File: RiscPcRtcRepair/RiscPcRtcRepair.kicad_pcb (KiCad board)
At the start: 2 copper layers, 22.5 x 32 mm, 16 parts, among them U1 PCF8583T, Y1 Crystal_GND3

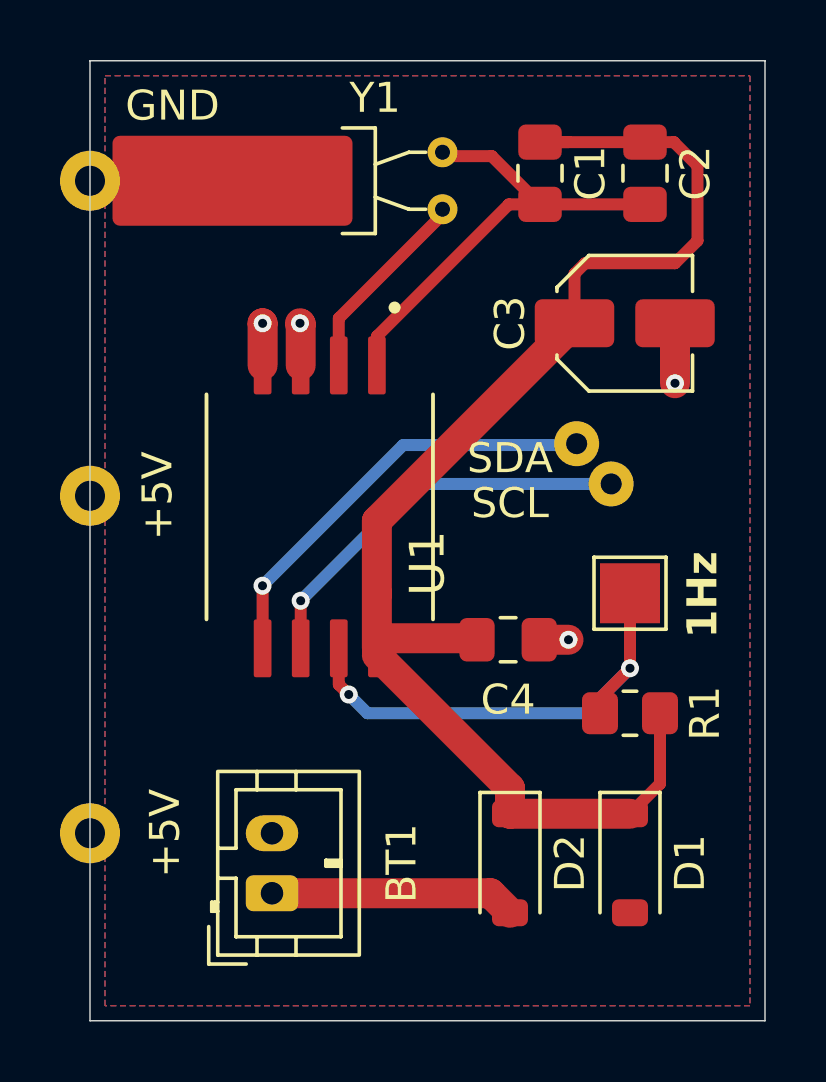
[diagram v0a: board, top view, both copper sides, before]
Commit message: Fix warnings and add gerbers
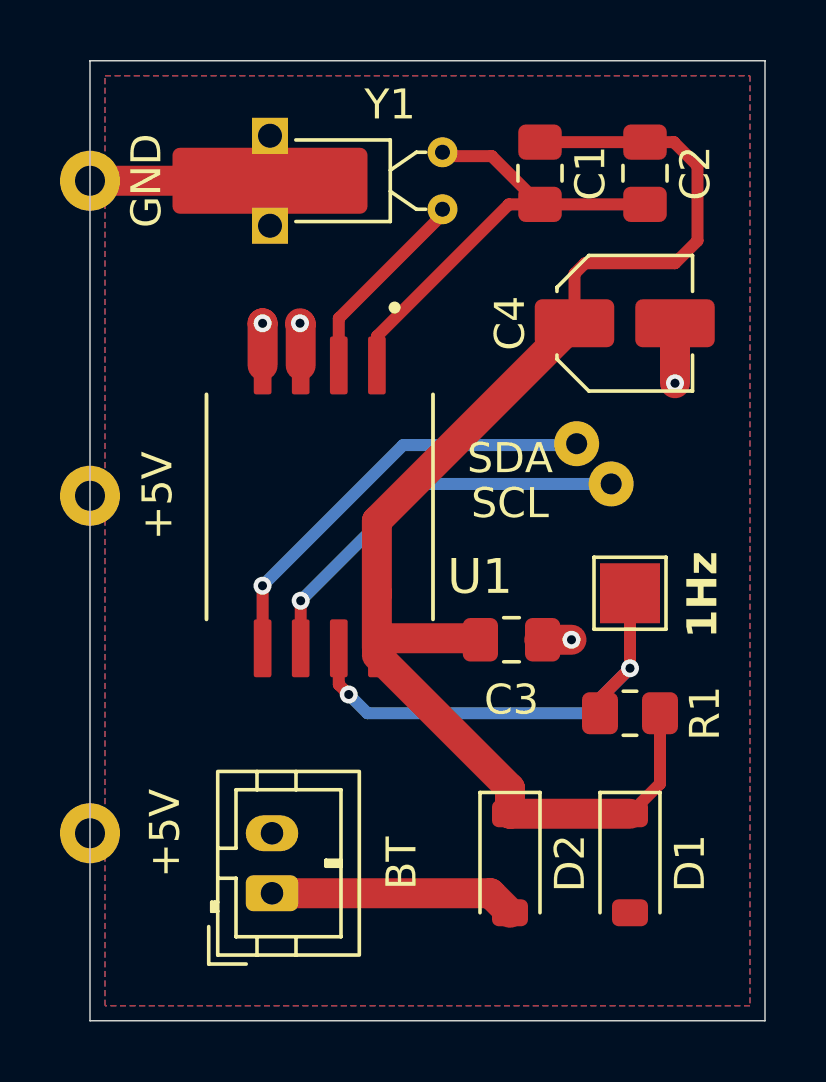
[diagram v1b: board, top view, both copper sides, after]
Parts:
- Y1: footprint Crystal:Crystal_C38-LF_D3.0mm_L8.0mm_Horizontal_1EP_style1 -> Crystal:Crystal_C26-LF_D2.1mm_L6.5mm_Horizontal_1EP_style2
- moved C3 0.11 mm to (107.0, 86.0)
- renumbered +5V2 to +5V1, BT1 to BT, C4 to C3, C3 to C4
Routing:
- net GND: track 5.80 -> 11.1 mm
- net Net-(D1-K): track 48.2 -> 47.2 mm
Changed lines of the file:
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@@
 		(tags "test point THT pad")
 		(property "Reference" "GND"
-			(at 2.75 -2.5 0)
+			(at 1.881715 0 90)
 			(layer "F.SilkS")
 			(effects
@@
 			(pinfunction "1")
 			(pintype "passive")
+			(zone_connect 2)
 		)
 		(embedded_fonts no)
@@
 		(descr "SMD capacitor, aluminum electrolytic nonpolar, 4.0x5.4mm")
 		(tags "capacitor electrolytic nonpolar")
-		(property "Reference" "C3"
+		(property "Reference" "C4"
 			(at -3.825 0 90)
 			(layer "F.SilkS")
@@
 		)
 	)
-	(footprint "Crystal:Crystal_C38-LF_D3.0mm_L8.0mm_Horizontal_1EP_style1"
+	(footprint "Crystal:Crystal_C26-LF_D2.1mm_L6.5mm_Horizontal_1EP_style2"
 		(layer "F.Cu")
 		(at 104.75 69.8 -90)
-		(descr "C38-LF, Crystal, length 8.0mm, width 3.0mm, THT")
+		(descr "C26-LF, Crystal, length 6.5mm, width 2.1mm, THT")
 		(property "Reference" "Y1"
-			(at -1.81 2.25 0)
+			(at -1.59 1.75 0)
 			(layer "F.SilkS")
 			(effects
@@
 		)
 		(property "Value" "Crystal_GND3"
-			(at 3.71 2.25 0)
+			(at 3.49 1.75 0)
 			(layer "F.Fab")
 			(effects
@@
 			)
 		)
-		(property "Datasheet" "~"
-			(at 0 0 90)
+		(property "Datasheet" ""
+			(at 0 0 270)
 			(layer "F.Fab")
 			(hide yes)
@@
 			)
 		)
-		(property "Description" "Three pin crystal, GND on pin 3"
-			(at 0 0 90)
+		(property "Description" ""
+			(at 0 0 270)
 			(layer "F.Fab")
 			(hide yes)
@@
 		(attr through_hole)
 		(fp_line
-			(start -0.81 3.34)
-			(end -0.81 2.24)
+			(start -0.41 4.89)
+			(end -0.41 1.74)
 			(stroke
 				(width 0.12)
@@
 		)
 		(fp_line
-			(start -0.81 2.24)
-			(end 2.71 2.24)
+			(start -0.41 1.74)
+			(end 2.31 1.74)
 			(stroke
 				(width 0.12)
@@
 		)
 		(fp_line
-			(start 0.405 2.24)
-			(end 0 1.12)
+			(start 0.6 1.74)
+			(end 0 0.87)
 			(stroke
 				(width 0.12)
@@
 		)
 		(fp_line
-			(start 1.495 2.24)
-			(end 1.9 1.12)
+			(start 1.3 1.74)
+			(end 1.9 0.87)
 			(stroke
 				(width 0.12)
@@
 		)
 		(fp_line
-			(start 2.71 2.24)
-			(end 2.71 3.34)
+			(start 2.31 1.74)
+			(end 2.31 4.89)
 			(stroke
 				(width 0.12)
@@
 		)
 		(fp_line
-			(start 0 1.12)
+			(start 0 0.87)
 			(end 0 0.56)
 			(stroke
@@
 		)
 		(fp_line
-			(start 1.9 1.12)
+			(start 1.9 0.87)
 			(end 1.9 0.56)
 			(stroke
@@
 		)
 		(fp_rect
-			(start -1.3 -0.75)
-			(end 3.2 11.25)
+			(start -1.4 -0.75)
+			(end 3.3 9.25)
 			(stroke
 				(width 0.05)
@@
 		)
 		(fp_line
-			(start 0.405 2.5)
-			(end 0 1.25)
+			(start -0.55 5.75)
+			(end 2.45 5.75)
 			(stroke
 				(width 0.1)
@@
 		)
 		(fp_line
-			(start 1.495 2.5)
-			(end 1.9 1.25)
+			(start 0.6 2)
+			(end 0 1)
 			(stroke
 				(width 0.1)
@@
 		)
 		(fp_line
-			(start 0 1.25)
+			(start 1.3 2)
+			(end 1.9 1)
+			(stroke
+				(width 0.1)
+				(type solid)
+			)
+			(layer "F.Fab")
+		)
+		(fp_line
+			(start 0 1)
 			(end 0 0)
 			(stroke
@@
 		)
 		(fp_line
-			(start 1.9 1.25)
+			(start 1.9 1)
 			(end 1.9 0)
 			(stroke
@@
 		)
 		(fp_rect
-			(start -0.55 2.5)
-			(end 2.45 10.5)
+			(start -0.08 2)
+			(end 1.98 8.5)
 			(stroke
 				(width 0.1)
@@
 		)
 		(fp_text user "${REFERENCE}"
-			(at 0.95 6.45 0)
+			(at 0.95 5.25 0)
 			(layer "F.Fab")
 			(effects
@@
 			(pintype "passive")
 		)
+		(pad "3" thru_hole rect
+			(at -0.55 5.75 270)
+			(size 1.2 1.2)
+			(drill 0.8)
+			(layers "*.Cu" "*.Mask")
+			(remove_unused_layers no)
+			(net 2 "GND")
+			(pinfunction "3")
+			(pintype "passive")
+		)
 		(pad "3" smd roundrect
-			(at 0.95 7 270)
-			(size 3 8)
+			(at 0.95 5.75 270)
+			(size 2.2 6.5)
 			(layers "F.Cu" "F.Mask" "F.Paste")
-			(roundrect_rratio 0.083333)
+			(roundrect_rratio 0.113636)
+			(net 2 "GND")
+			(pinfunction "3")
+			(pintype "passive")
+		)
+		(pad "3" thru_hole rect
+			(at 2.45 5.75 270)
+			(size 1.2 1.2)
+			(drill 0.8)
+			(layers "*.Cu" "*.Mask")
+			(remove_unused_layers no)
 			(net 2 "GND")
 			(pinfunction "3")
@@
 		)
 		(embedded_fonts no)
-		(model "${KICAD9_3DMODEL_DIR}/Crystal.3dshapes/Crystal_C38-LF_D3.0mm_L8.0mm_Horizontal_1EP_style1.step"
+		(model "${KICAD9_3DMODEL_DIR}/Crystal.3dshapes/Crystal_C26-LF_D2.1mm_L6.5mm_Horizontal_1EP_style2.step"
 			(offset
 				(xyz 0 0 0)
@@
 		(descr "JST PH series connector, B2B-PH-K (http://www.jst-mfg.com/product/pdf/eng/ePH.pdf), generated with kicad-footprint-generator")
 		(tags "connector JST PH vertical")
-		(property "Reference" "BT1"
+		(property "Reference" "BT"
 			(at 1 4.318777 90)
 			(layer "F.SilkS")
@@
 			(pinfunction "-")
 			(pintype "passive")
+			(zone_connect 2)
 		)
 		(embedded_fonts no)
@@
 		(descr "THT pad as test Point, diameter 2.0mm, hole diameter 1.0mm")
 		(tags "test point THT pad")
-		(property "Reference" "+5V2"
+		(property "Reference" "+5V1"
 			(at 1.5 -3 90)
 			(layer "F.SilkS")
@@
 		(at 100.658166 81.620968 -90)
 		(property "Reference" "U1"
-			(at 1.879032 -3.591834 270)
+			(at 2.329032 -5.341834 0)
 			(layer "F.SilkS")
 			(effects
@@
 	(footprint "Capacitor_SMD:C_0805_2012Metric_Pad1.18x1.45mm_HandSolder"
 		(layer "F.Cu")
-		(at 106.9375 86.05 180)
+		(at 107.05 86.05 180)
 		(descr "Capacitor SMD 0805 (2012 Metric), square (rectangular) end terminal, IPC-7351 nominal with elongated pad for handsoldering. (Body size source: IPC-SM-782 page 76, https://www.pcb-3d.com/wordpress/wp-content/uploads/ipc-sm-782a_amendment_1_and_2.pdf, https://docs.google.com/spreadsheets/d/1BsfQQcO9C6DZCsRaXUlFlo91Tg2WpOkGARC1WS5S8t0/edit?usp=sharing), generated with kicad-footprint-generator")
 		(tags "capacitor handsolder")
-		(property "Reference" "C4"
+		(property "Reference" "C3"
 			(at 0 -2 0)
 			(layer "F.SilkS")
@@
 	)
 	(segment
-		(start 100.023166 76.905968)
-		(end 100.023166 75.523166)
+		(start 107.975 86.05)
+		(end 109.05 86.05)
 		(width 1)
 		(layer "F.Cu")
@@
 	)
 	(segment
-		(start 107.975 86.05)
-		(end 108.95 86.05)
+		(start 99 70.75)
+		(end 93.8 70.75)
+		(width 1)
+		(layer "F.Cu")
+		(net 2)
+	)
+	(segment
+		(start 100.023166 76.905968)
+		(end 100.023166 75.523166)
 		(width 1)
 		(layer "F.Cu")
@@
 	)
 	(via
-		(at 108.95 86.05)
+		(at 100 75.5)
 		(size 0.6)
 		(drill 0.3)
@@
 	)
 	(via
-		(at 100 75.5)
+		(at 109.05 86.05)
 		(size 0.6)
 		(drill 0.3)
@@
 	(segment
 		(start 102.563166 82.086834)
-		(end 109.15 75.5)
+		(end 102.563166 84.5)
 		(width 1)
 		(layer "F.Cu")
@@
 	)
 	(segment
-		(start 105.7875 86)
-		(end 102.563166 86)
+		(start 102.563166 82.086834)
+		(end 109.15 75.5)
 		(width 1)
 		(layer "F.Cu")
@@
 	)
 	(segment
-		(start 108 69.4625)
-		(end 108.9625 69.4625)
-		(width 0.4)
+		(start 105.7875 86)
+		(end 102.563166 86)
+		(width 1)
 		(layer "F.Cu")
 		(net 4)
@@
 	)
 	(segment
-		(start 102.600666 84.4625)
-		(end 102.563166 84.5)
-		(width 0.4)
-		(layer "F.Cu")
-		(net 4)
-	)
-	(segment
 		(start 102.563166 86.563166)
 		(end 107 91)
 		(width 1)
 		(layer "F.Cu")
-		(net 4)
-	)
-	(segment
-		(start 102.563166 84.5)
-		(end 102.563166 82.086834)
-		(width 1)
-		(layer "F.Cu")
